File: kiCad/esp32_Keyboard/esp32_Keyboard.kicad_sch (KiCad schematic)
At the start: 171 parts, among them SW1 Switch, SW10 Switch, SW11 Switch, SW12 Switch, SW13 Switch, SW14 Switch, SW15 Switch, SW16 Switch, SW17 Switch, SW18 Switch, SW19 Switch, SW2 Switch, SW20 Switch, SW21 Switch, SW22 Switch, SW23 Switch, SW24 Switch, SW25 Switch, SW26 Switch, SW27 Switch, SW28 Switch, SW29 Switch, SW3 Switch, SW30 Switch, SW31 Switch, SW32 Switch, SW33 Switch, SW34 Switch, SW35 Switch, SW36 Switch, SW37 Switch, SW38 Switch, SW39 Switch, SW4 Switch, SW40 Switch, SW41 Switch, SW42 Switch, SW43 Switch, SW44 Switch, SW45 Switch, SW46 Switch, SW47 Switch, SW48 Switch, SW49 Switch, SW5 Switch, SW50 Switch, SW51 Switch, SW52 Switch, SW53 Switch, SW54 Switch, SW55 Switch, SW56 Switch, SW57 Switch, SW58 Switch, SW59 Switch, SW6 Switch, SW60 Switch, SW61 Switch, SW62 Switch, SW63 Switch, SW64 Switch, SW65 Switch, SW66 Switch, SW67 Switch, SW68 Switch, SW69 Switch, SW7 Switch, SW70 Switch, SW71 Switch, SW72 Switch, SW73 Switch, SW74 Switch, SW75 Switch, SW76 Switch, SW77 Switch, SW78 Switch, SW79 Switch, SW8 Switch, SW80 Switch, SW81 Switch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

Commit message: finished layout circuit baord V1
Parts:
- removed R1: 10K, ScottoKeebs_Components:Resistor_0402, symbol ScottoKeebs:Placeholder_Resistor
- added Dsp1: ~, tigmitLib:GC9A01 roundDisplay Footprint, symbol tigmitSymbolLib:GC9A01_Round_Display
- added J1, J2: Conn_01x15, Connector_PinHeader_2.54mm:PinHeader_1x15_P2.54mm_Vertical, symbol Connector_Generic:Conn_01x15
- added R2, R3, R4, R5, R6, R7: 10K, Resistor_THT:R_Axial_DIN0204_L3.6mm_D1.6mm_P7.62mm_Horizontal, symbol ScottoKeebs:Placeholder_Resistor
- added U4: ~, tigmitLib:b103 multichannel fader pot, symbol tigmitSymbolLib:b013_dual_channel_sliding_pot
- added U5: ESP32-DEVKIT-V1 DisplayHandler, ESP32-DEVKIT-V1:MODULE_ESP32_DEVKIT_V1, symbol ESP32-DEVKIT-V1:ESP32-DEVKIT-V1
- SW1, SW10, SW11, SW12, SW13, SW14, SW15, SW16, SW17, SW18, SW19, SW2, SW20, SW21, SW22, SW23, SW24, SW25, SW26, SW27, SW29, SW3, SW31, SW32, SW33, SW34, SW35, SW36, SW37, SW38, SW39, SW4, SW40, SW41, SW42, SW44, SW46, SW47, SW48, SW49, SW5, SW50, SW51, SW52, SW53, SW54, SW55, SW56, SW59, SW6, SW60, SW61, SW62, SW63, SW64, SW65, SW66, SW67, SW68, SW7, SW70, SW79, SW8, SW80, SW81, SW9: footprint ScottoKeebs_MX:MX_PCB_1.00u -> ScottoKeebs_Hotswap:Hotswap_MX_1.00u
- SW28: footprint ScottoKeebs_MX:MX_PCB_2.00u -> ScottoKeebs_Hotswap:Hotswap_MX_2.00u
- SW30, SW43: footprint ScottoKeebs_MX:MX_PCB_1.50u -> ScottoKeebs_Hotswap:Hotswap_MX_1.50u
- SW45: footprint ScottoKeebs_MX:MX_PCB_1.75u -> ScottoKeebs_Hotswap:Hotswap_MX_1.75u
- SW57, SW58: footprint ScottoKeebs_MX:MX_PCB_2.25u -> ScottoKeebs_Hotswap:Hotswap_MX_2.25u
- SW69: footprint ScottoKeebs_MX:MX_PCB_2.75u -> ScottoKeebs_Hotswap:Hotswap_MX_2.75u
- SW71, SW72, SW73, SW75, SW76, SW77, SW78: footprint ScottoKeebs_MX:MX_PCB_1.25u -> ScottoKeebs_Hotswap:Hotswap_MX_1.25u
- SW74: footprint ScottoKeebs_MX:MX_PCB_6.25u -> ScottoKeebs_Hotswap:Hotswap_MX_6.25u
- U1: value ESP32-DEVKIT-V1 -> ESP32-DEVKIT-V1 Matrix Handler
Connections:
- net GND: now also U2.13 (~{OE}), U3.13 (~{OE}), Dsp1.2 (GND), J1.2 (Pin_2), J2.14 (Pin_14), R2.2, R3.2, R4.2, R5.2, R6.2, R7.2, U4.6, U4.7 (mount), U5.2 (GND), U5.29 (GND)
- net Row0: now also U1.19 (D34), R2.1; no longer U1.21 (D32)
- net Row1: now also U1.20 (D35), R3.1; no longer U1.25 (D27)
- net Row2: now also U1.21 (D32), R4.1; no longer U1.24 (D26)
- net Row3: now also U1.22 (D33), R5.1; no longer U1.23 (D25)
- net Row4: now also U1.23 (D25), R6.1; no longer U1.15 (D23)
- net Row5: now also U1.24 (D26), R7.1; no longer U1.14 (D22)
- net VCC: now also U2.10 (~{SRCLR}), U3.10 (~{SRCLR}), Dsp1.1 (vcc), J2.15 (Pin_15), U4.3, U5.1 (3V3)
- net at U1.12 (RX0): now also J2.4 (Pin_4)
- net at U1.13 (TX0): now also J2.3 (Pin_3)
- net at U1.16 (EN): now also J1.15 (Pin_15)
- net at U1.17 (VP): now also J1.14 (Pin_14)
- net at U1.18 (VN): now also J1.13 (Pin_13)
- net at U1.26 (D14): now also J1.5 (Pin_5)
- net at U1.27 (D12): now also J1.4 (Pin_4)
- net RCLK / LATCH: now reaches U1.28 (D13)
- net RCLK / LATCH: now also U2.12 (RCLK), U3.12 (RCLK)
- net at U1.30 (VIN): now also J1.1 (Pin_1)
- net at U1.4 (D2): now also J2.12 (Pin_12)
- net at U1.5 (D4): now also J2.11 (Pin_11)
- net at U1.6 (RX2): now also J2.10 (Pin_10)
- net at U1.7 (TX2): now also J2.9 (Pin_9)
- net at U1.8 (D5): now also J2.8 (Pin_8)
- removed net RCLK: U1.10 (D19), U2.11 (SRCLK), U2.12 (RCLK), U3.11 (SRCLK), U3.12 (RCLK)
- net SER renamed SER / DATA
- net SER / DATA: now also U1.15 (D23); no longer U1.11 (D21)
- removed net /OE: U1.3 (D15), U2.13 (~{OE}), U3.13 (~{OE})
- removed net /SRCLR: U1.9 (D18), U2.10 (~{SRCLR}), U3.10 (~{SRCLR})
- new net: J1.6 (Pin_6), U1.25 (D27)
- new net: J2.6 (Pin_6), U1.10 (D19)
- new net: J2.13 (Pin_13), U1.3 (D15)
- new net DSP  SDA: Dsp1.4 (SDA), U5.15 (D23)
- new net DSP CS: Dsp1.6 (CS), J2.2 (Pin_2), U1.14 (D22), U5.14 (D22)
- new net DSP DC: Dsp1.5 (DC), U5.6 (RX2)
- new net DSP RST: Dsp1.7 (RST), U5.5 (D4)
- new net DSP SCL: Dsp1.3 (SCL), U5.9 (D18)
- new net POT slider Pin: U4.4
- new net SRCLK / CLOCK: U1.9 (D18), U2.11 (SRCLK), U3.11 (SRCLK)
- new net esp32-SDA: J2.5 (Pin_5), U1.11 (D21), U5.11 (D21)
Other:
- note removed: "for now WIP"
- note removed: "might need to pull /OE low throug 10k Res"
- moved on the sheet: U1, U2, U3

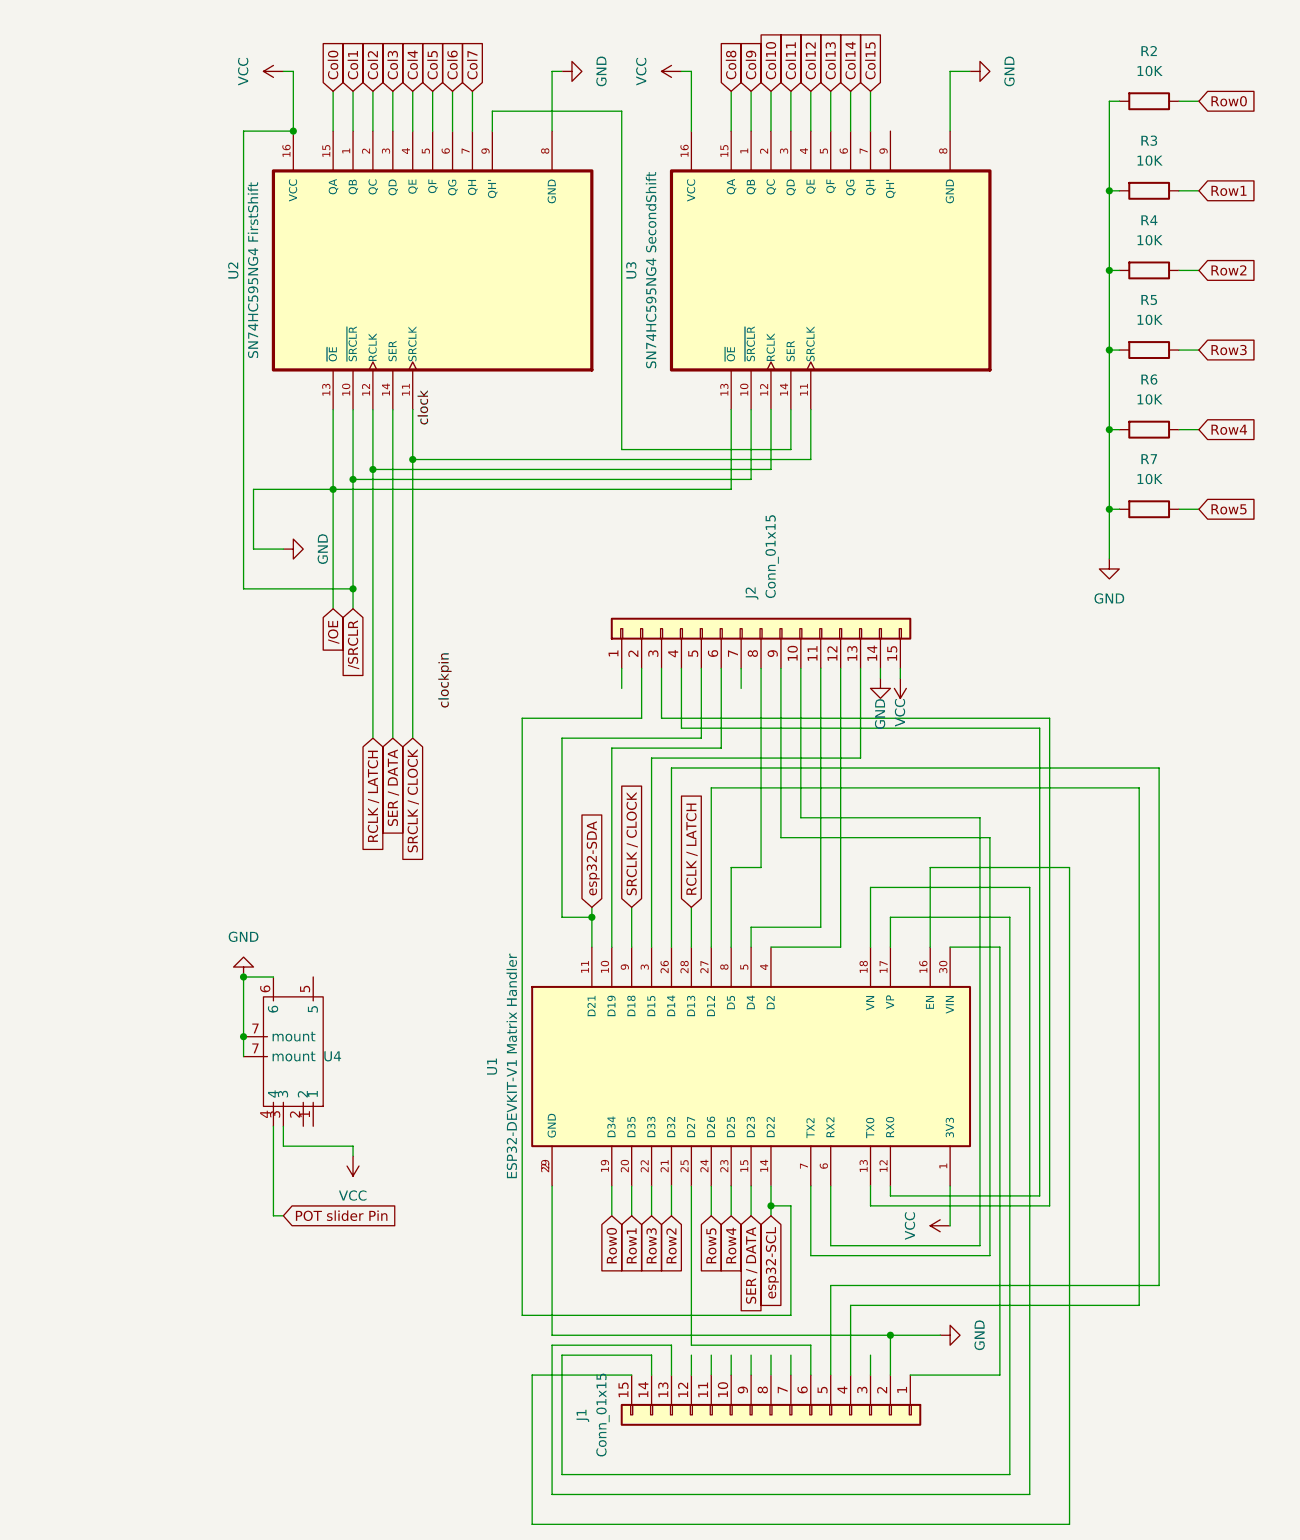
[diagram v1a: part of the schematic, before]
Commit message: finished PCB design
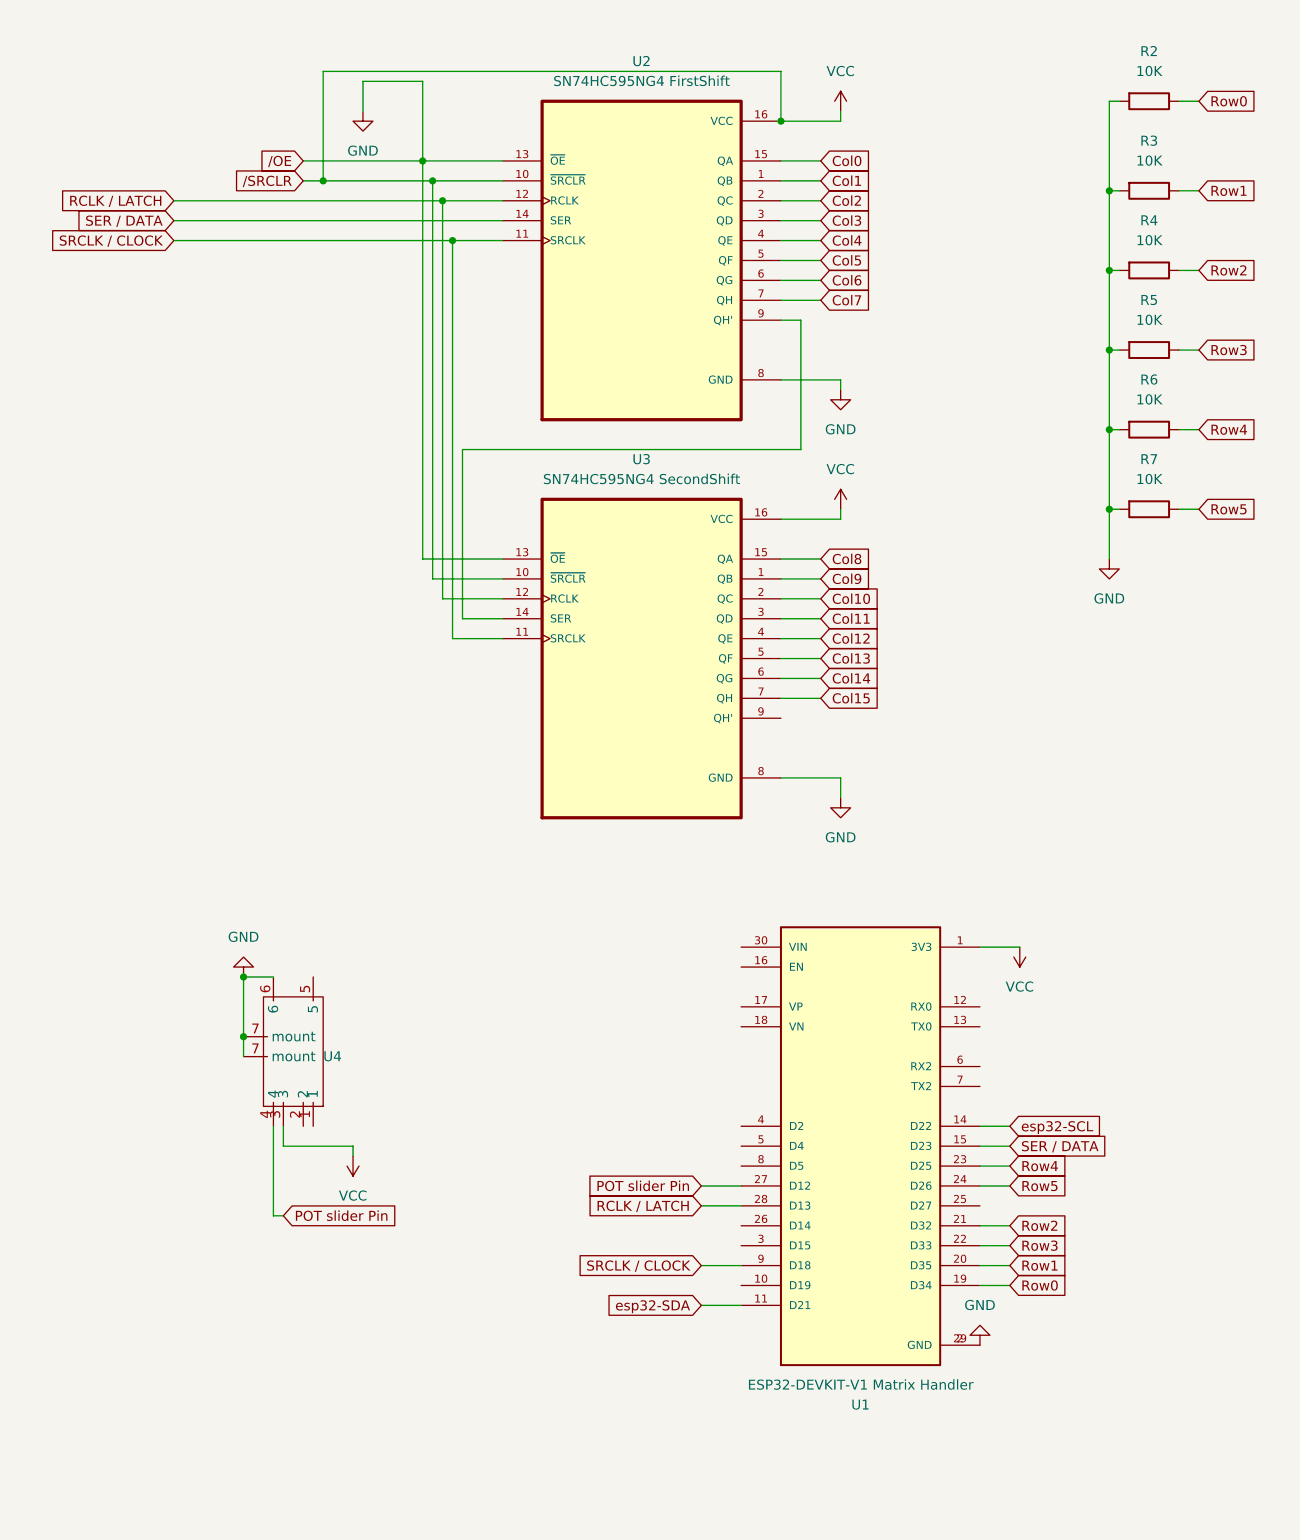
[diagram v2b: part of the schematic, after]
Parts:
- removed J1, J2: Conn_01x15, Connector_PinHeader_2.54mm:PinHeader_1x15_P2.54mm_Vertical, symbol Connector_Generic:Conn_01x15
- Dsp1: footprint tigmitLib:GC9A01 roundDisplay Footprint -> Connector_PinHeader_2.54mm:PinHeader_1x07_P2.54mm_Vertical
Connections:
- net POT slider Pin: now also U1.27 (D12)
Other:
- moved on the sheet: U1, U2, U3
